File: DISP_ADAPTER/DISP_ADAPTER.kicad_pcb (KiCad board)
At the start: 2 copper layers, 2 parts, among them J1 FH12-40S-0.5SH(55), J2 Conn_02x20_Odd_Even

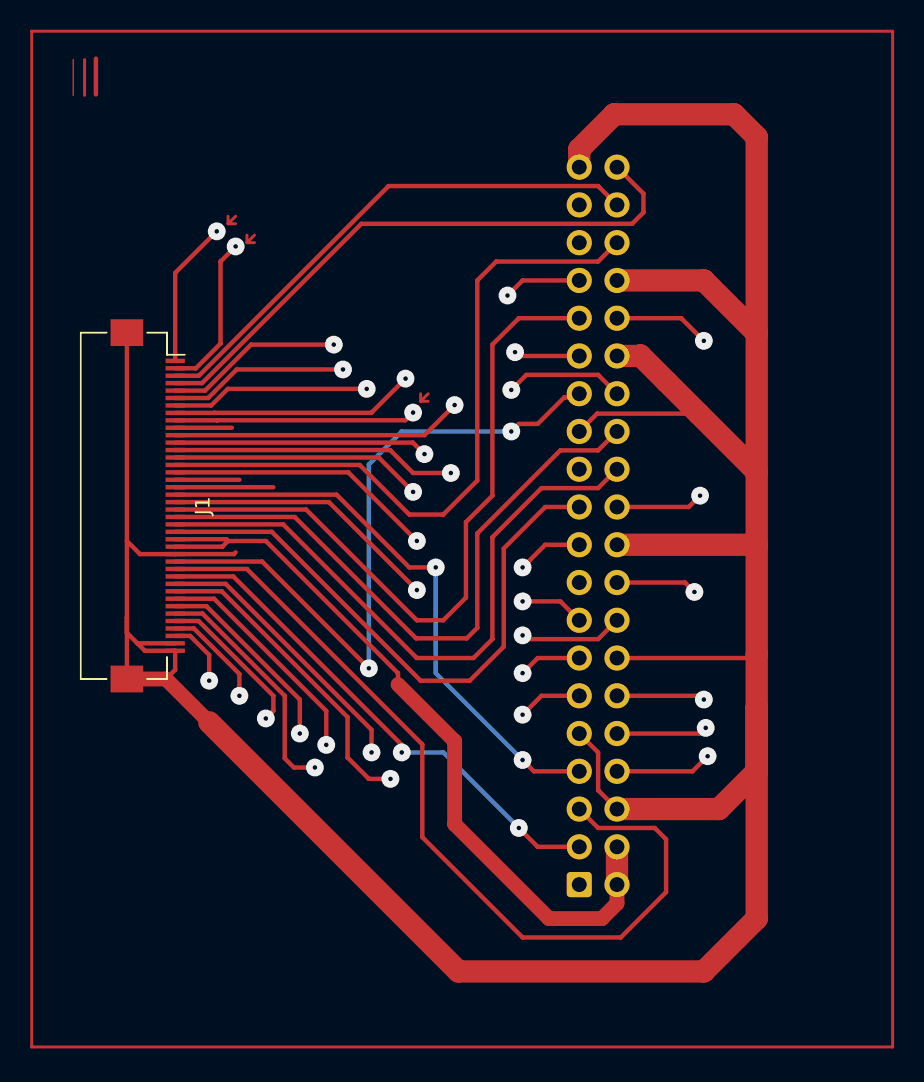
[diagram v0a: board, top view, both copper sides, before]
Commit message: PWM set
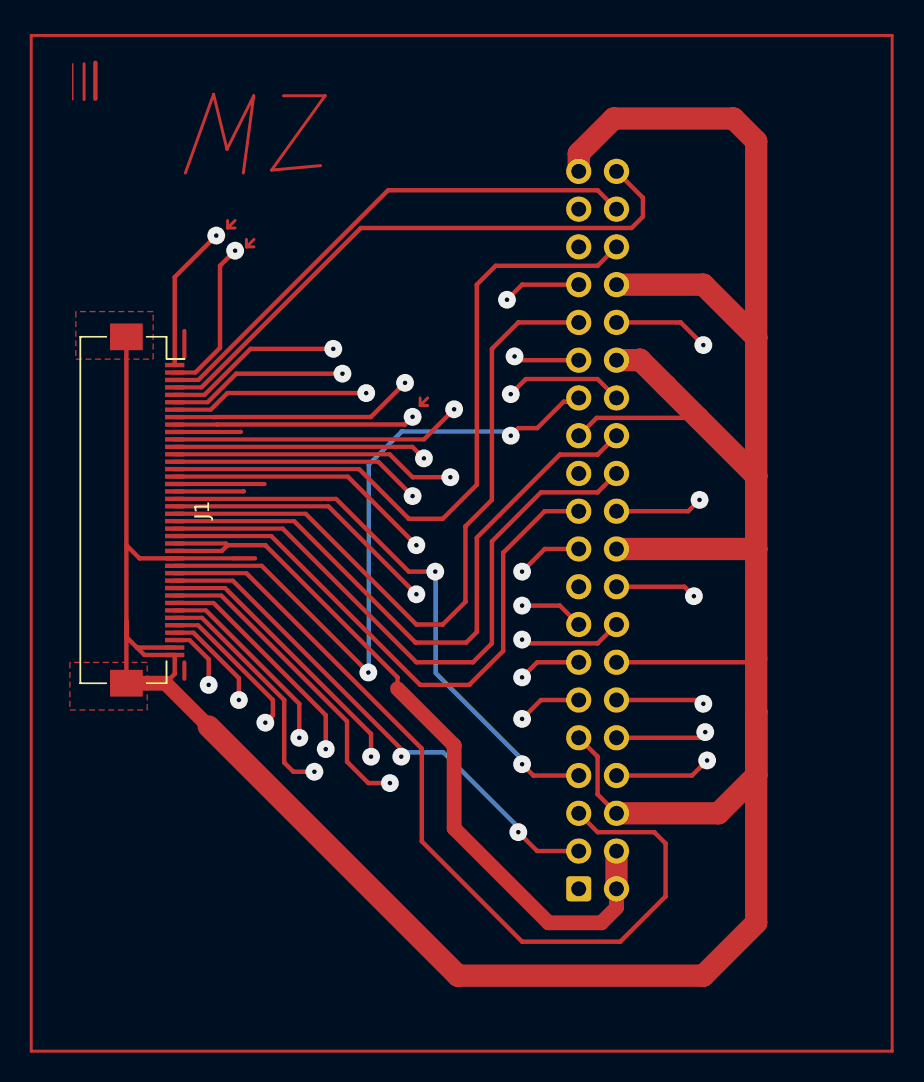
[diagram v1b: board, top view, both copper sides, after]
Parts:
- moved J2 0.29 mm to (51.5, 76.2)
- moved J1 0.29 mm to (22.5, 50.8)
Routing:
- net (no net): track 0.00 -> 2.90 mm
- net /LCD_B1: track 6.60 -> 4.66 mm
- net /LCD_B0: track 4.32 -> 6.05 mm
- net GND: track 231.7 -> 233.0 mm
- net /LCD_G1: track 3.81 -> 4.46 mm
- added copper zone on F.Cu, net GND
